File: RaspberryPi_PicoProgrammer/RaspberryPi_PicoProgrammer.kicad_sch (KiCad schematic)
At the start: 7 parts, among them J1 Conn_02x05_Odd_Even, J2 Conn_01x07_Male, J3 Conn_02x03_Odd_Even, J4 BM03B-SRSS-TBLFSN, U1 Pico

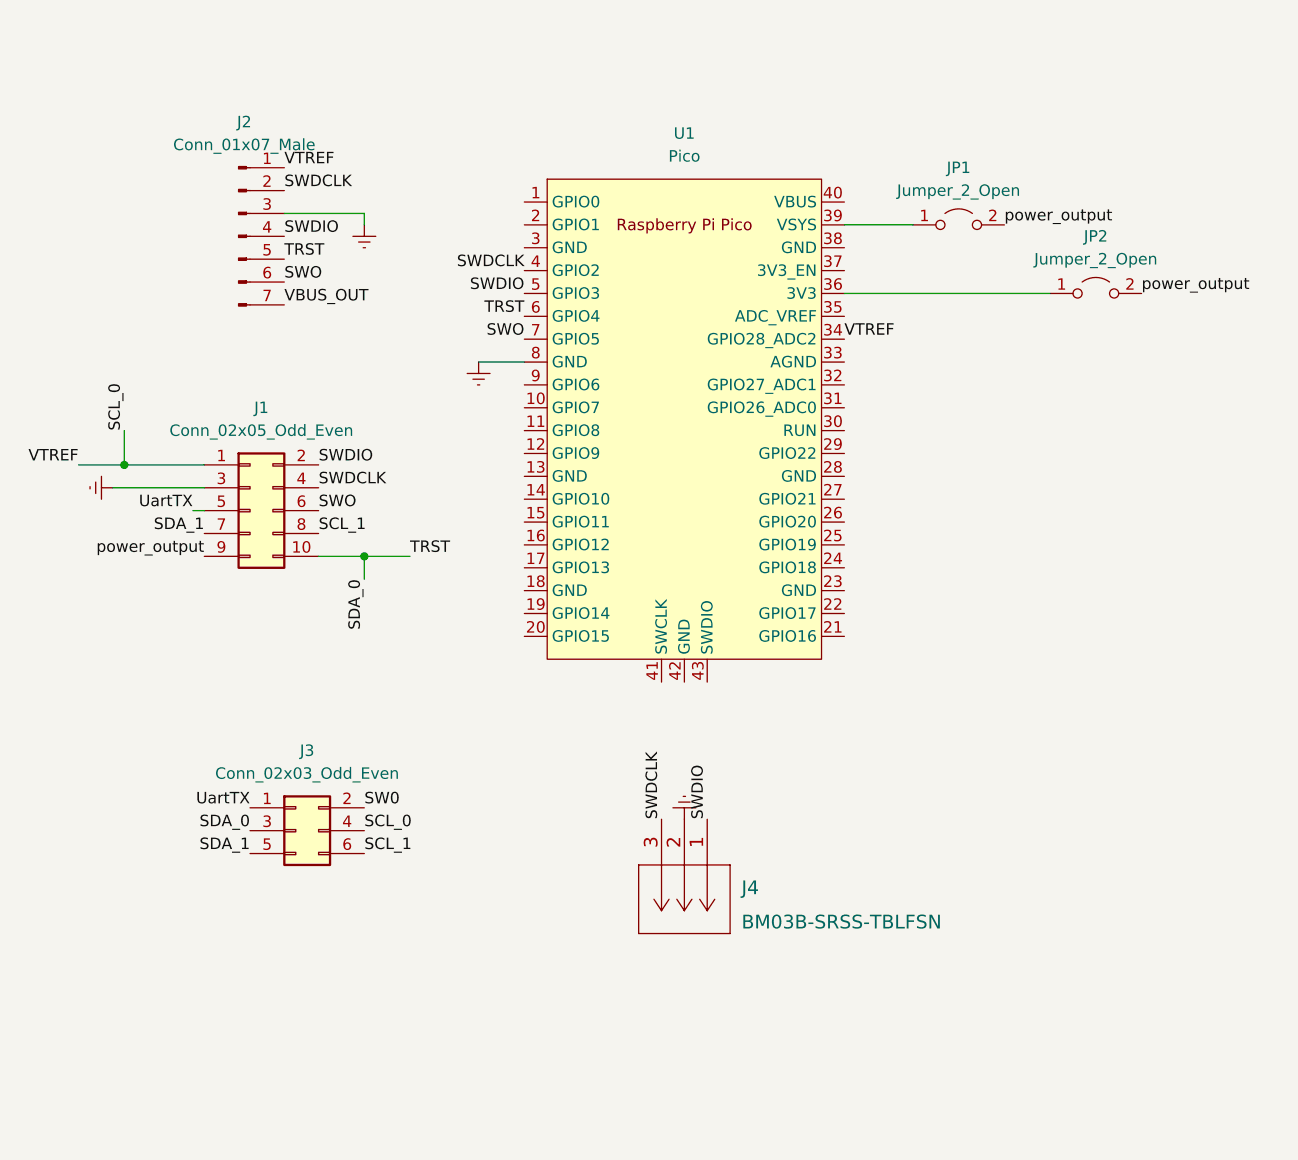
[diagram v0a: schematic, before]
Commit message: added schematic for raspberry pi
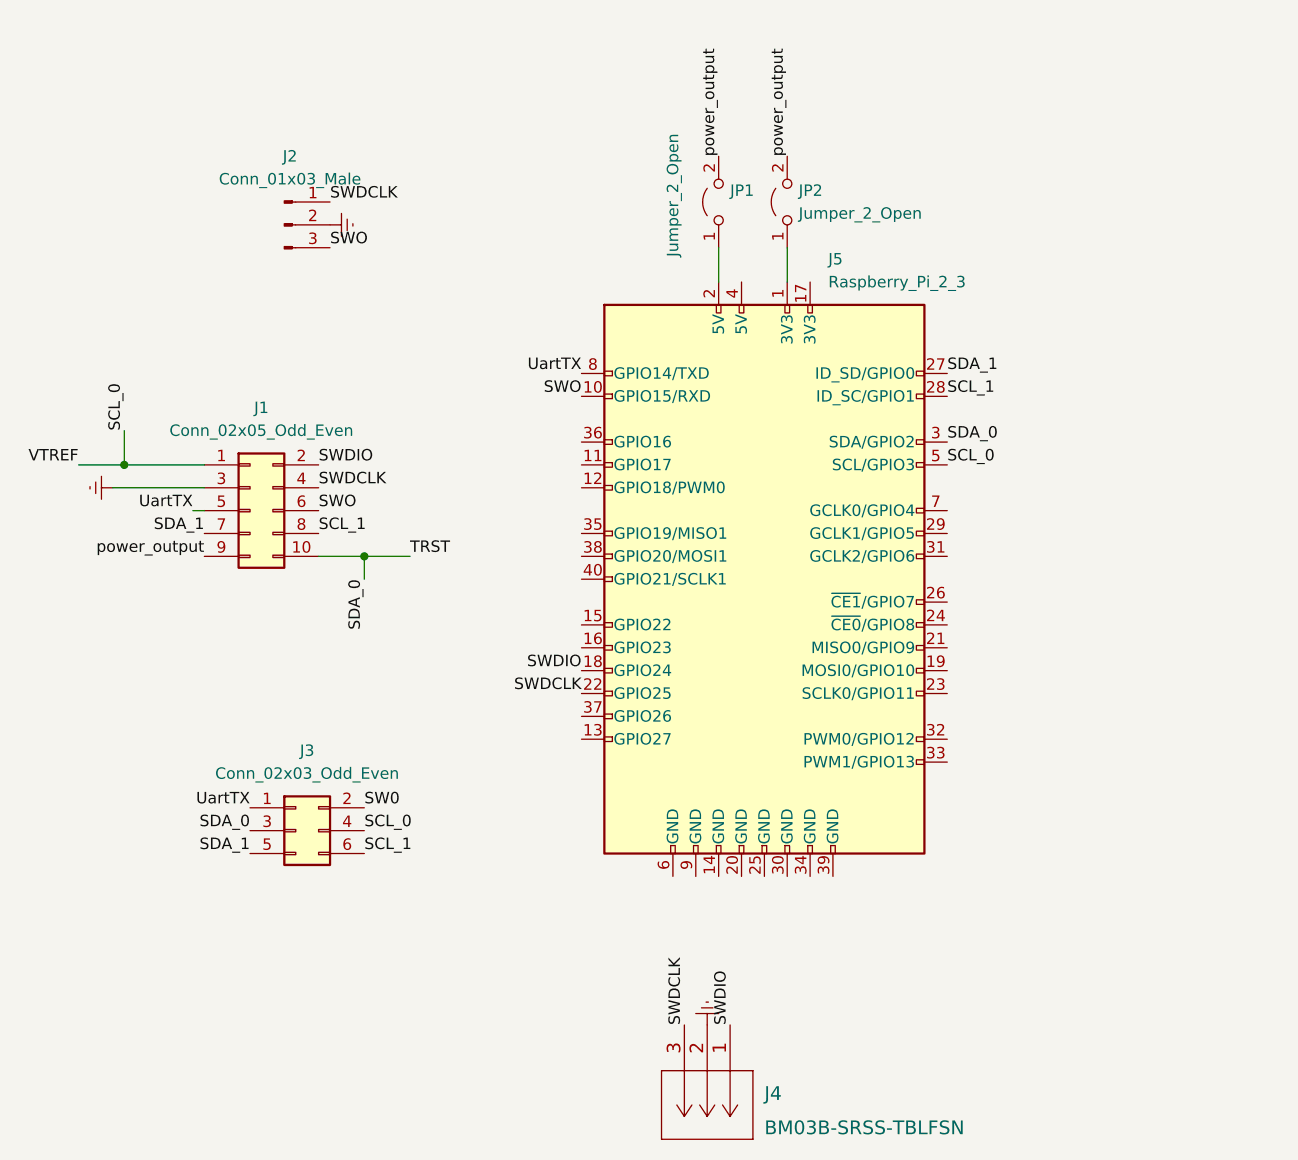
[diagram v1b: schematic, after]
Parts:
- removed J2: Conn_01x07_Male, Connector_PinSocket_2.54mm:PinSocket_1x07_P2.54mm_Horizontal, symbol Connector:Conn_01x07_Male
- removed U1: Pico, MCU_RaspberryPi_and_Boards:RPi_Pico_SMD_TH, symbol MCU_RaspberryPi_and_Boards:Pico
- added J2: Conn_01x03_Male, Connector_PinHeader_2.54mm:PinHeader_1x03_P2.54mm_Horizontal, symbol Connector:Conn_01x03_Male
- added J5: Raspberry_Pi_2_3, Connector_PinHeader_2.54mm:PinHeader_2x20_P2.54mm_Vertical, symbol Connector:Raspberry_Pi_2_3
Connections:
- net Earth: now also J2.2 (Pin_2)
- net SCL_0: now also J5.5 (SCL/GPIO3)
- net SCL_1: now also J5.28 (ID_SC/GPIO1)
- net SDA_0: now also J5.3 (SDA/GPIO2)
- net SDA_1: now also J5.27 (ID_SD/GPIO0)
- net SWDCLK: now also J2.1 (Pin_1), J5.22 (GPIO25)
- net SWDIO: now also J5.18 (GPIO24)
- net SWO: now also J2.3 (Pin_3), J5.10 (GPIO15/RXD)
- net UartTX: now also J5.8 (GPIO14/TXD)
- net at JP1.1 (A): now also J5.2 (5V)
- net at JP2.1 (A): now also J5.1 (3V3)
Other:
- moved on the sheet: J4, JP1, JP2
